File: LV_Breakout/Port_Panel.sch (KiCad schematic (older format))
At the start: 36 parts, among them J1 171-009-113R911, J10 TE 776228-1, J11 2.54mmPins, J2 B3B-PH-K-S(LF)(SN), J3 Conn_02x03_Odd_Even, J4 171-009-213R001, J5 USB_B, J6 RJ45, J7 B6B-XH-A(LF)(SN), J8 B12B-PUDSS-1(LF)(SN), J9 RJ45, Q1 PSMN5R2-60YL, Q2 PSMN5R2-60YL, U1 ATmega328P-AU, U2 MCP2515-xSO, U3 MCP2551-I-SN, U4 MAX232, Y1 16MHz

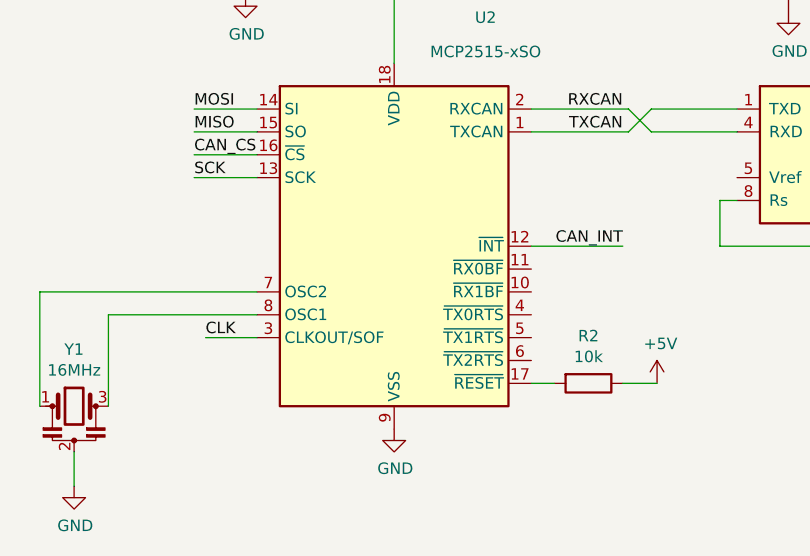
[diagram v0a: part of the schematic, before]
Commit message: minor updates
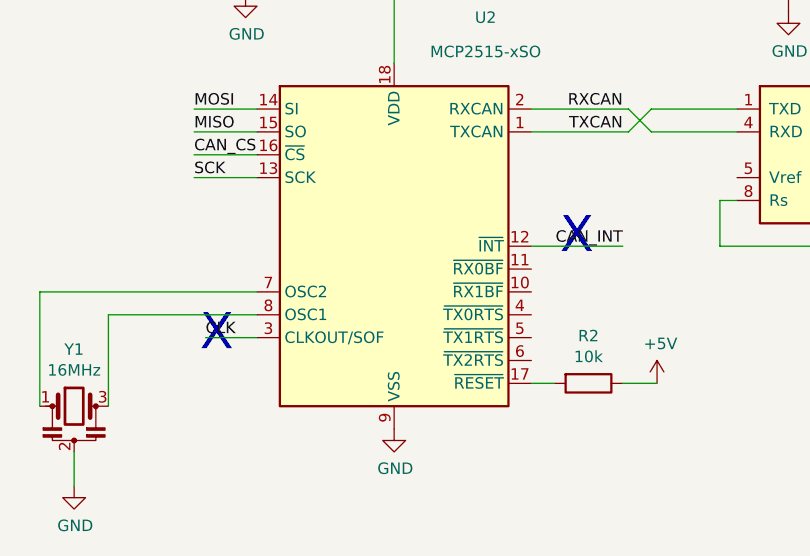
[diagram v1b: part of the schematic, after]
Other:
- note added: "X"
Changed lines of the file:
@@
 Text Notes 10950 1325 0    50   ~ 0
 Sensor_4
+Text Notes 3475 6425 0    157  ~ 0
+X
+Text Notes 1900 6850 0    157  ~ 0
+X
 $EndSCHEMATC
